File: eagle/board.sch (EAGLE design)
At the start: 31 parts

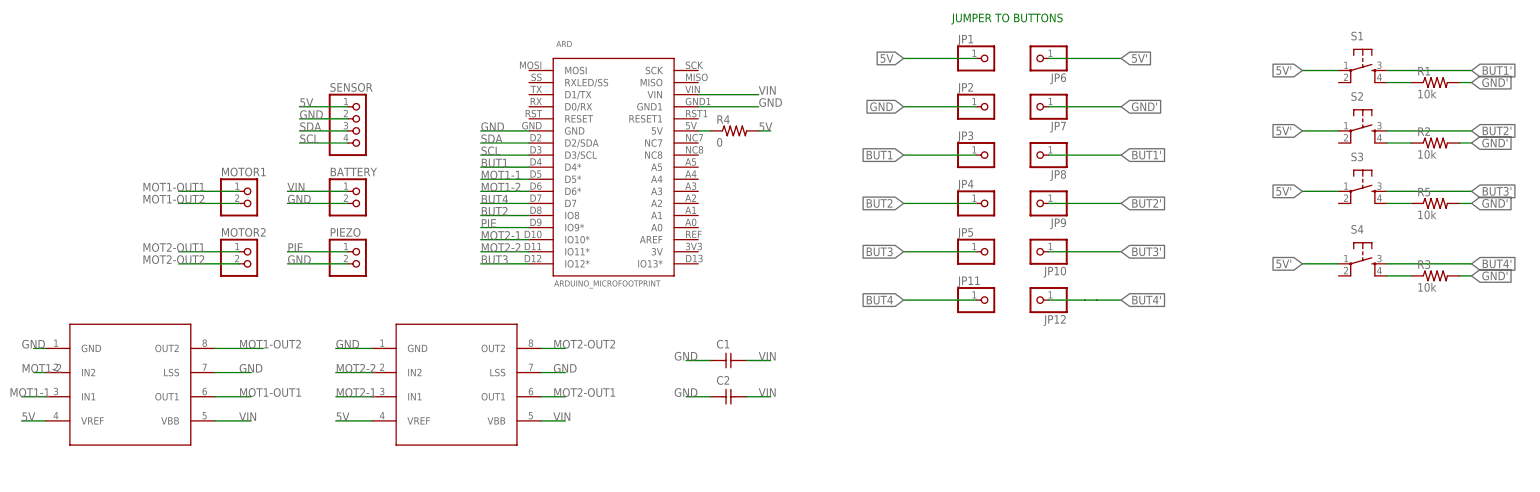
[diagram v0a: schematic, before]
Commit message: pcb update
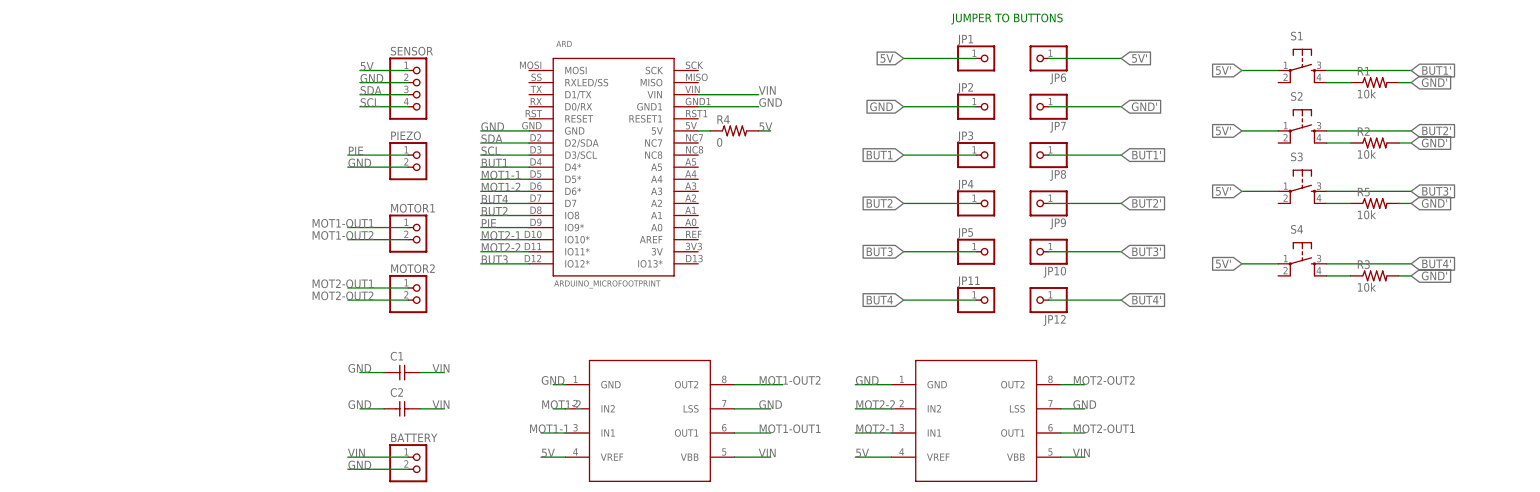
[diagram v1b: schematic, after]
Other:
- moved on the sheet: BATTERY, C1, C2, MOTOR1, MOTOR2, PIEZO, R1, R2, R3, R5, S1, S2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
